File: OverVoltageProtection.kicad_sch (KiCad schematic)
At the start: 18 parts, among them Q3 IRFR210PBF, Q4 IRFR210PBF, U1 LM74800QDRRRQ1, U2 LM5069MM-2_NOPB

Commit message: sample layout
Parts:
- added C1: 1uF, symbol PCM_Elektuur:C
- added C7: 150nF, symbol PCM_Elektuur:C
- added C8: 330uF, symbol PCM_Elektuur:C
- added D5: SMBJ30A-13-F, SMBJ30A-13-F:DIOM5336X250N, symbol SMBJ30A-13-F:SMBJ30A-13-F
- added D6: SS310, Diode_SMD:D_SMA, symbol Diode:SS310
- added Q1: IRFR210PBF, Package_TO_SOT_SMD:TO-252-3_TabPin2, symbol Device:Q_NMOS_Depletion_GDS
- added R1, R4: 47.5k, symbol PCM_Elektuur:R
- added R10: 100k, symbol PCM_Elektuur:R
- added R2: 8.25k, symbol PCM_Elektuur:R
- added R7: 4.22k, symbol PCM_Elektuur:R
- added R8: 0.004R, symbol PCM_Elektuur:R
- added R9: 15.8k, symbol PCM_Elektuur:R
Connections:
- net OUT is gone; now on net V_FILTERED: C6.1 (+), D4.2 (A), Q3.3 (S), Q4.3 (S), U1.2 (A), U1.9 (OUT)
- net GND: now also U2.5 (GND), C1.2 (-), C7.2 (-), C8.2 (-), D5.2, D6.2 (A), R2.2 (-), R7.2 (-), R9.2 (-)
- net VOUT: now also U2.2 (VIN), C1.1 (+), D5.1, R1.1 (+), R4.1 (+), R8.1 (+)
- net SENSE: now reaches U2.1 (SENSE)
- net SENSE: now also Q1.2 (D), R8.2 (-)
- net at U2.10 (GATE): now also Q1.1 (G)
- net UVLO: now reaches U2.3 (UVLO)
- net UVLO: now also R1.2 (-), R2.1 (+)
- net at U2.4 (OVLO): now also R4.2 (-), R7.1 (+)
- net at U2.6 (TIMER): now also C7.1 (+)
- net at U2.7 (PWR): now also R9.1 (+)
- net PGOOD: now reaches U2.8 (PGD)
- net PGOOD: now also R10.2 (-)
- net V_FILTERED: now reaches U2.9 (OUT)
- net V_FILTERED: now also C8.1 (+), D6.1 (K), Q1.3 (S)
- new net +5V: R10.1 (+)
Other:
- moved on the sheet: C2, C3, C4, C5, C6, D1, D2, D3, D4, JP1, JP2, Q3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

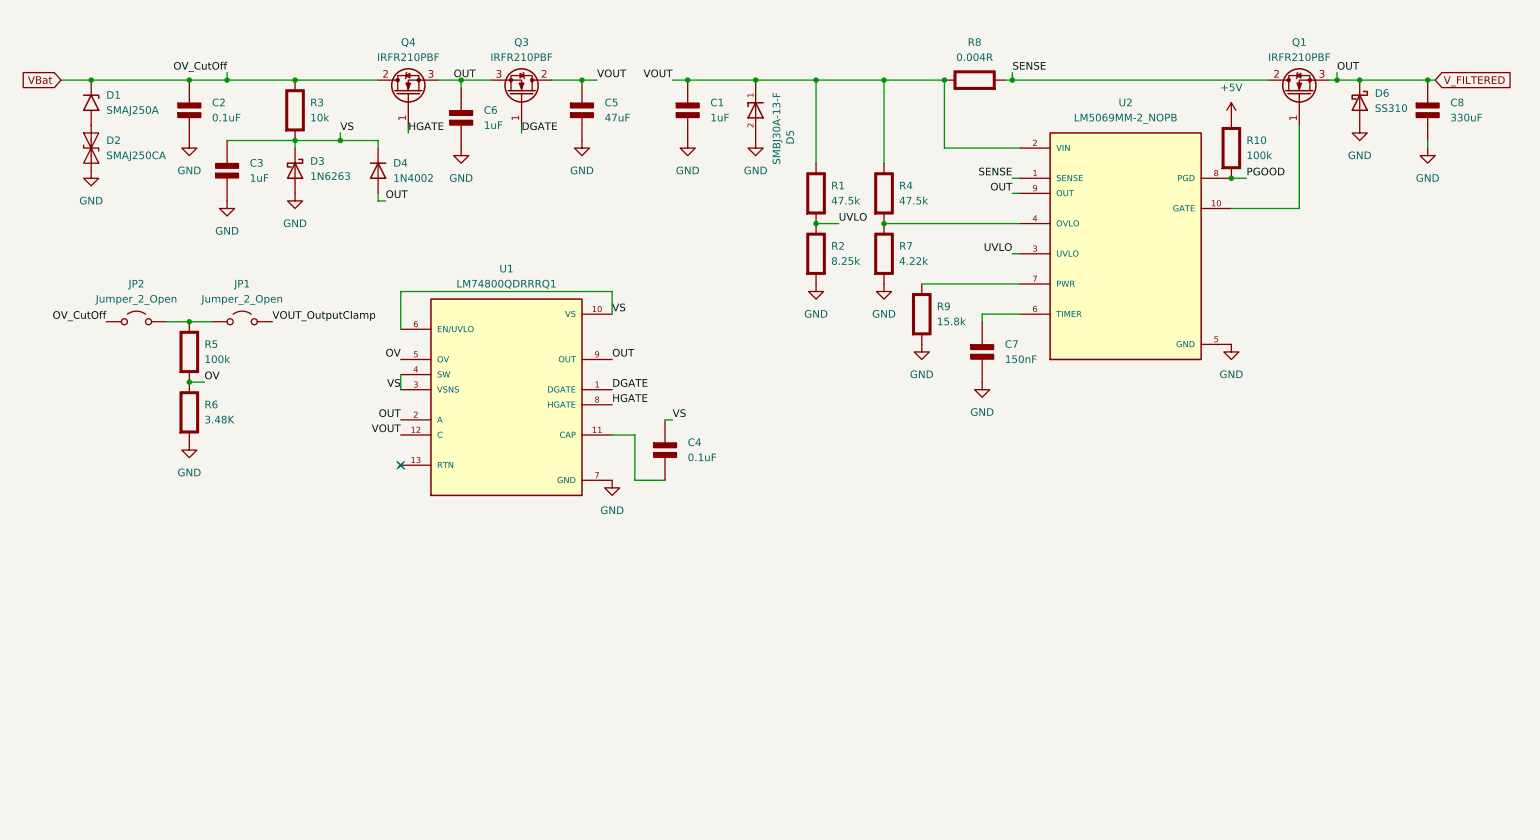
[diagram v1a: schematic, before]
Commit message: prototyple schematics finished
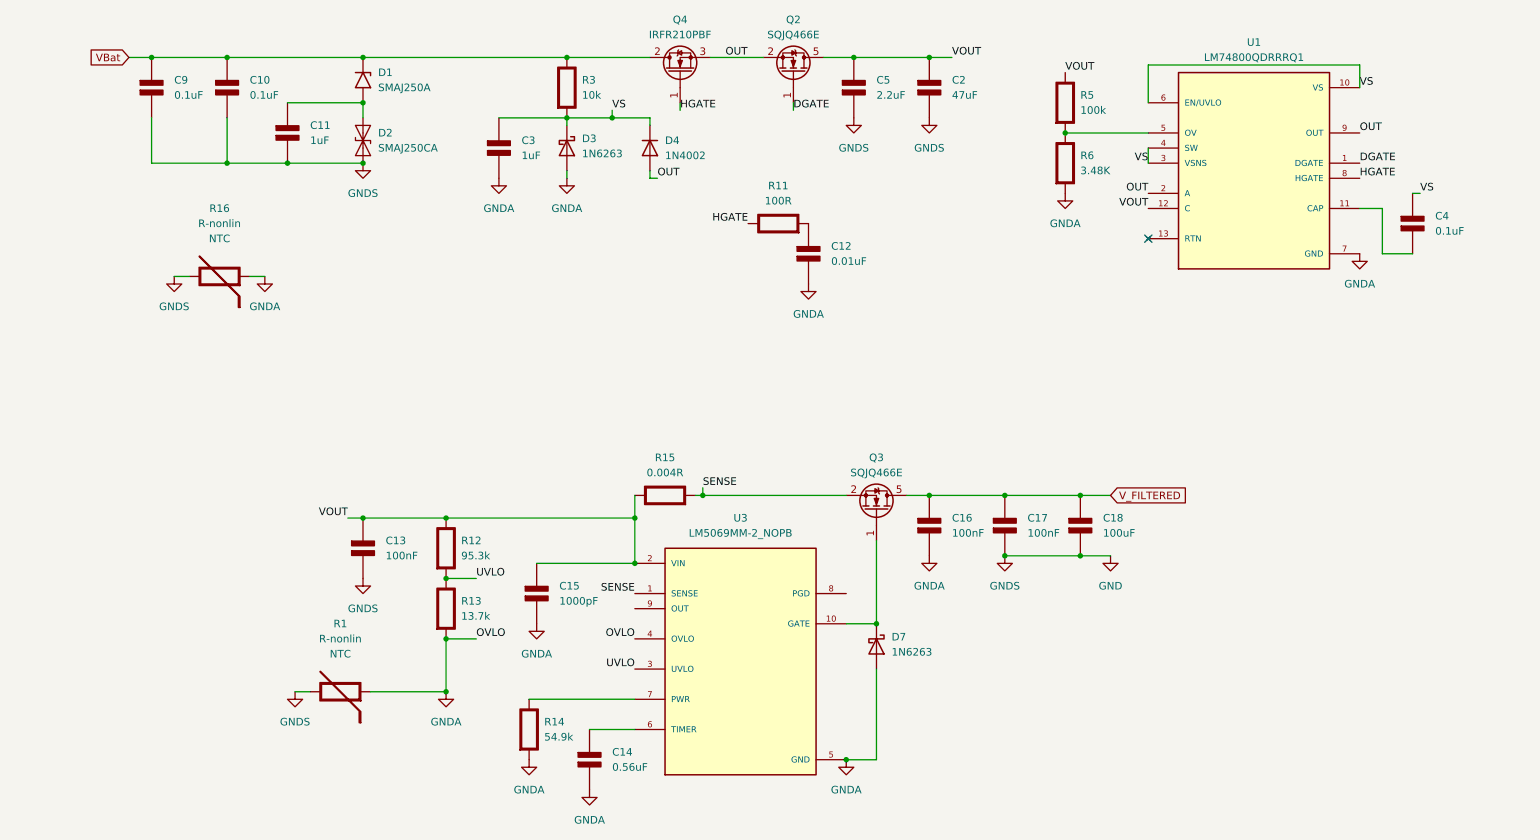
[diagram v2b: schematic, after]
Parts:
- removed C1, C6: 1uF, symbol PCM_Elektuur:C
- removed C7: 150nF, symbol PCM_Elektuur:C
- removed C8: 330uF, symbol PCM_Elektuur:C
- removed D5: SMBJ30A-13-F, SMBJ30A-13-F:DIOM5336X250N, symbol SMBJ30A-13-F:SMBJ30A-13-F
- removed D6: SS310, Diode_SMD:D_SMA, symbol Diode:SS310
- removed JP1, JP2: Jumper_2_Open, symbol Jumper:Jumper_2_Open
- removed Q1, Q3: IRFR210PBF, Package_TO_SOT_SMD:TO-252-3_TabPin2, symbol Device:Q_NMOS_Depletion_GDS
- removed R1, R4: 47.5k, symbol PCM_Elektuur:R
- removed R10: 100k, symbol PCM_Elektuur:R
- removed R2: 8.25k, symbol PCM_Elektuur:R
- removed R7: 4.22k, symbol PCM_Elektuur:R
- removed R8: 0.004R, symbol PCM_Elektuur:R
- removed R9: 15.8k, symbol PCM_Elektuur:R
- removed U2: LM5069MM-2_NOPB, LM5069MM-2_NOPB:SOP50P490X110-10N, symbol LM5069MM-2_NOPB:LM5069MM-2_NOPB
- added C10, C9: 0.1uF, symbol PCM_Elektuur:C
- added C11: 1uF, symbol PCM_Elektuur:C
- added C12: 0.01uF, symbol PCM_Elektuur:C
- added C13, C16, C17: 100nF, symbol PCM_Elektuur:C
- added C14: 0.56uF, symbol PCM_Elektuur:C
- added C15: 1000pF, symbol PCM_Elektuur:C
- added C18: 100uF, symbol PCM_Elektuur:C
- added D7: 1N6263, Diode_THT:D_DO-35_SOD27_P7.62mm_Horizontal, symbol Diode:1N6263
- added Q2, Q3: SQJQ466E, Package_TO_SOT_SMD:LFPAK88, symbol Transistor_FET:SQJQ466E
- added R1, R16: R-nonlin, symbol PCM_Elektuur:R-nonlin
- added R11: 100R, symbol PCM_Elektuur:R
- added R12: 95.3k, symbol PCM_Elektuur:R
- added R13: 13.7k, symbol PCM_Elektuur:R
- added R14: 54.9k, symbol PCM_Elektuur:R
- added R15: 0.004R, symbol PCM_Elektuur:R
- added U3: LM5069MM-2_NOPB, LM5069MM-2_NOPB:SOP50P490X110-10N, symbol LM5069MM-2_NOPB:LM5069MM-2_NOPB
- C2: value 0.1uF -> 47uF
- C5: value 47uF -> 2.2uF
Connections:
- net DGATE: now also Q2.1 (G)
- net GND: now also C10.2 (-), C11.2 (-), C13.2 (-), C17.2 (-), C18.2 (-), C9.2 (-), R1.1 (+), R16.1 (+); no longer C3.2 (-), D3.2 (A), R6.2 (-), U1.7 (GND)
- net HGATE: now also R11.1 (+)
- net SENSE: now also Q3.2 (S), Q3.3 (S), Q3.4 (S), R15.2 (-), U3.1 (SENSE)
- net UVLO: now also R12.2 (-), R13.1 (+), U3.3 (UVLO)
- net VBat: now also C10.1 (+), C9.1 (+); no longer C2.1 (+)
- net VOUT: now also C2.1 (+), R5.1 (+), C13.1 (+), C15.1 (+), Q2.5 (D), R12.1 (+), R15.1 (+), U3.2 (VIN)
- net V_FILTERED: now also C16.1 (+), C17.1 (+), C18.1 (+), Q3.5 (D); no longer D4.2 (A), Q4.3 (S), U1.2 (A), U1.9 (OUT)
- net at D1.2 (A2), D2.2 (A2): now also C11.1 (+)
- net OV: no longer names the net of R5.2 (-), R6.1 (+), U1.5 (OV)
- new net: C12.1 (+), R11.2 (-)
- new net: R14.1 (+), U3.7 (PWR)
- new net: D7.1 (K), Q3.1 (G), U3.10 (GATE)
- new net: C14.1 (+), U3.6 (TIMER)
- new net GNDA: C12.2 (-), C14.2 (-), C15.2 (-), C16.2 (-), C3.2 (-), D3.2 (A), D7.2 (A), R1.2 (-), R13.2 (-), R14.2 (-), R16.2 (-), R6.2 (-), U1.7 (GND), U3.4 (OVLO), U3.5 (GND)
- new net OUT: D4.2 (A), Q2.2 (S), Q2.3 (S), Q2.4 (S), Q4.3 (S), U1.2 (A), U1.9 (OUT)
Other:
- moved on the sheet: C3, C4, C5, D1, D2, D3, D4, Q4, R3, R5, R6, U1
